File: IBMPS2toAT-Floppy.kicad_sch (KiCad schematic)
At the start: 3 parts

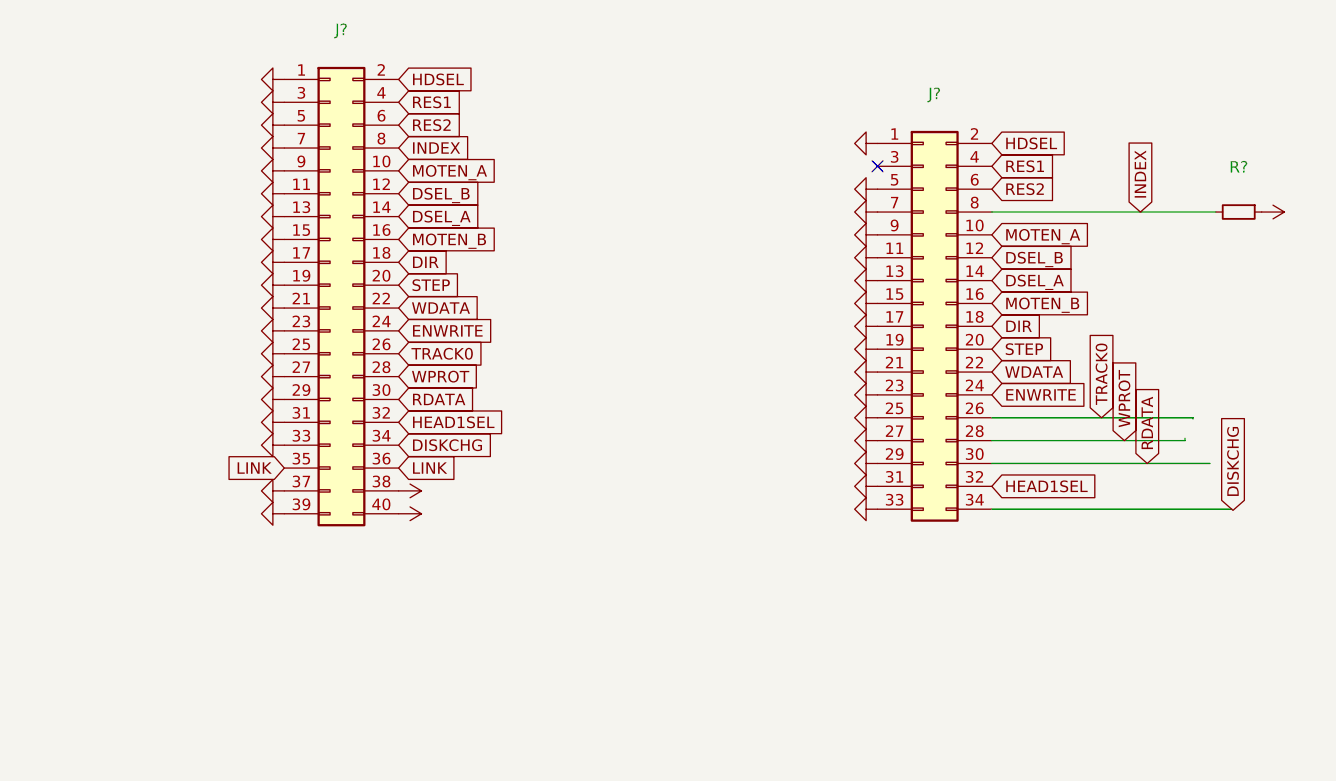
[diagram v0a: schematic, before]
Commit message: rev1
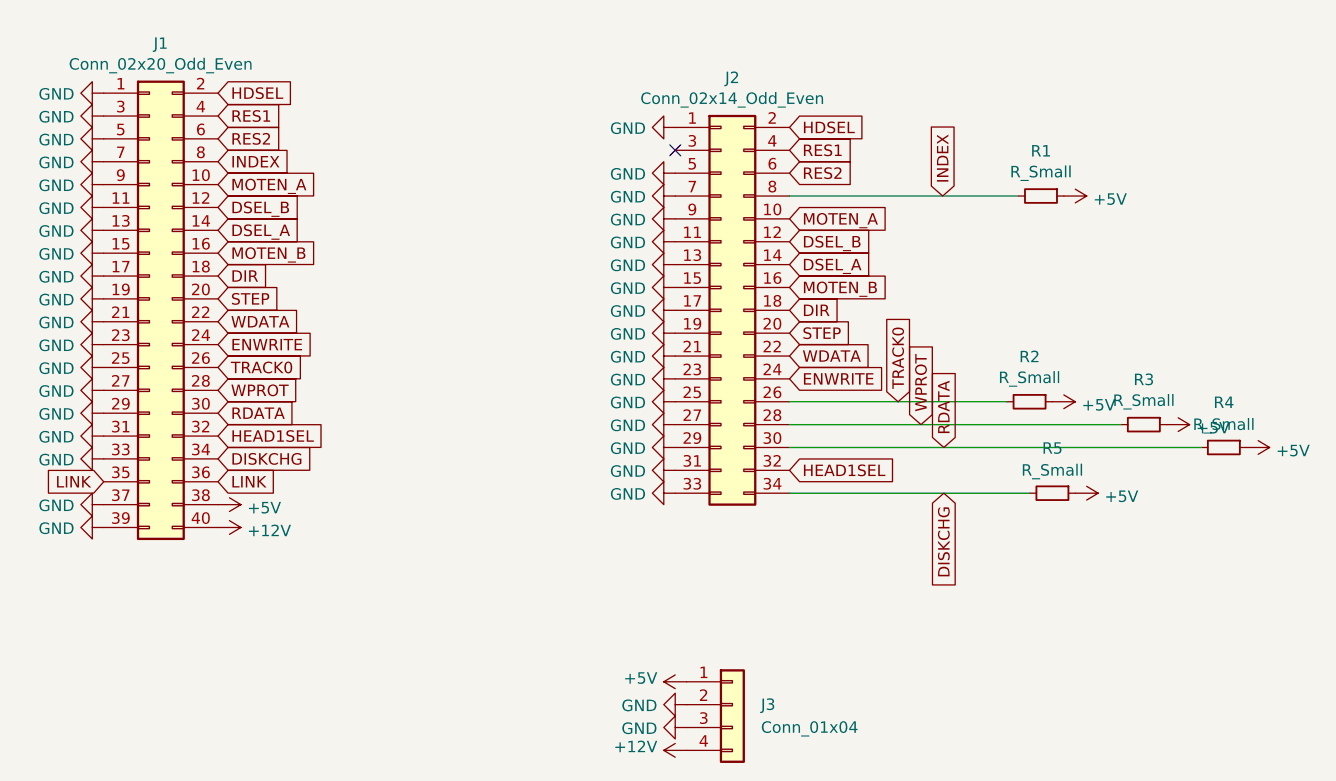
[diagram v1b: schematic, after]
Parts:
- added J3: Conn_01x04, Connector_JST:JST_XH_B4B-XH-A_1x04_P2.50mm_Vertical, symbol Connector_Generic:Conn_01x04
- added R1, R3, R4, R5: R_Small, Resistor_SMD:R_1206_3216Metric, symbol Device:R_Small
- J1: renamed from J?; value (none) -> Conn_02x20_Odd_Even; footprint (none) -> Sebs-footprints:IBM_2x20_EDGE
- J2: renamed from J?; value (none) -> Conn_02x14_Odd_Even; footprint (none) -> Connector_PinSocket_2.54mm:PinSocket_2x17_P2.54mm_Vertical
- R2: renamed from R?; value (none) -> R_Small; footprint (none) -> Resistor_SMD:R_1206_3216Metric
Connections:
- net +12V: now also J3.4 (Pin_4)
- net +5V: now also J3.1 (Pin_1), R1.1, R3.1, R4.1, R5.1
- net DISKCHG: now also J2.34 (Pin_34), R5.2
- net GND: now also J3.2 (Pin_2), J3.3 (Pin_3)
- net INDEX: now also R1.2; no longer R2.2
- net RDATA: now also R4.2
- net TRACK0: now also R2.2
- net WPROT: now also R3.2
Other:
- moved on the sheet: J1, J2, R2

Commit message: updates
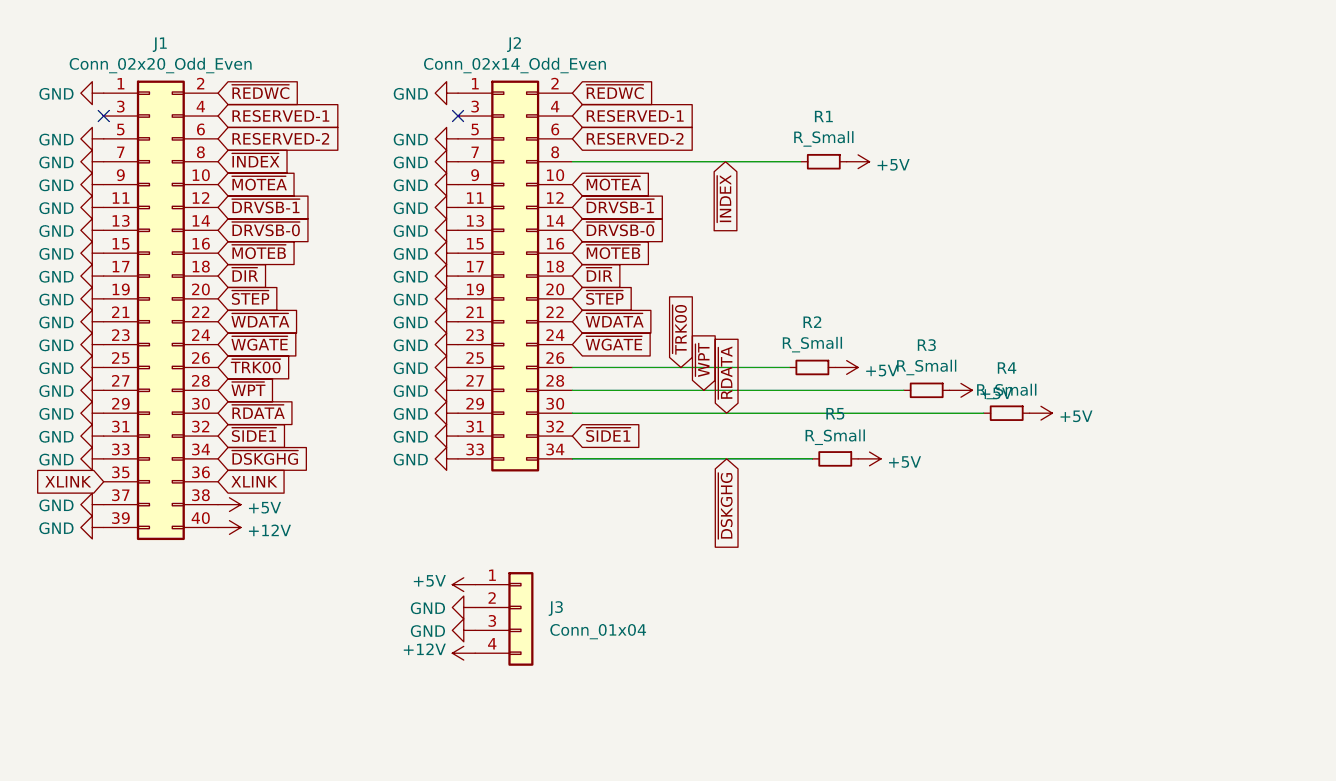
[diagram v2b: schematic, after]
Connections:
- net GND: no longer J1.3 (Pin_3)
- net DIR renamed ~{DIR}
- net DISKCHG renamed ~{DSKGHG}
- net DSEL_A renamed ~{DRVSB-0}
- net DSEL_B renamed ~{DRVSB-1}
- net ENWRITE renamed ~{WGATE}
- net HDSEL renamed ~{REDWC}
- net HEAD1SEL renamed ~{SIDE1}
- net INDEX renamed ~{INDEX}
- net LINK renamed XLINK
- net MOTEN_A renamed ~{MOTEA}
- net MOTEN_B renamed ~{MOTEB}
- net RDATA renamed ~{RDATA}
- net RES1 renamed RESERVED-1
- net RES2 renamed RESERVED-2
- net STEP renamed ~{STEP}
- net TRACK0 renamed ~{TRK00}
- net WDATA renamed ~{WDATA}
- net WPROT renamed ~{WPT}
- no-connect marks 1 -> 2
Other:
- moved on the sheet: J2, J3, R1, R2, R3, R4, R5
